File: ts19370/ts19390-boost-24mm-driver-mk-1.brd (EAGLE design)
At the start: 20 x 20 mm, 14 parts, among them U1 TINY85, U2 AMC7135SOT-89, U3 AMC7135SOT-89, U4 AMC7135SOT-89, U5 AMC7135SOT-89

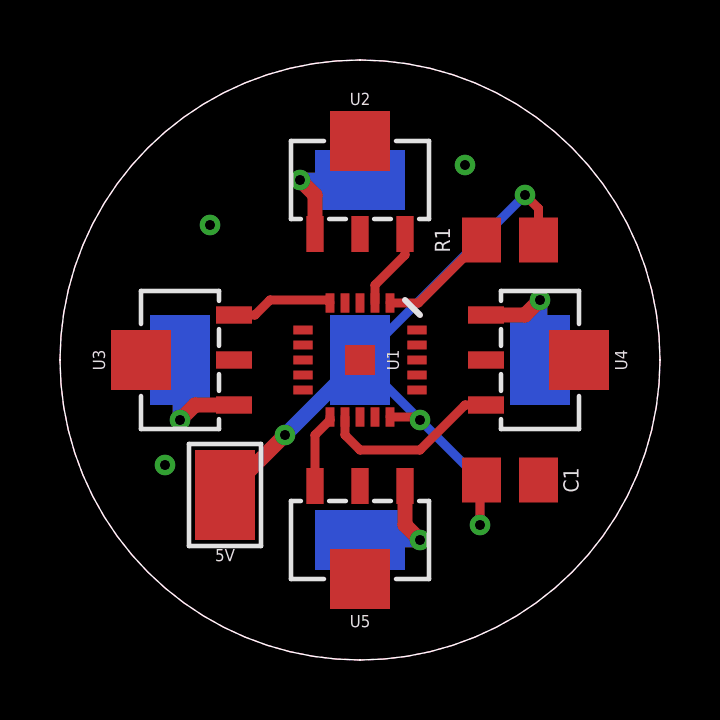
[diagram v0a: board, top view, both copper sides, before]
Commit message: faaaabulous flashlight in progress
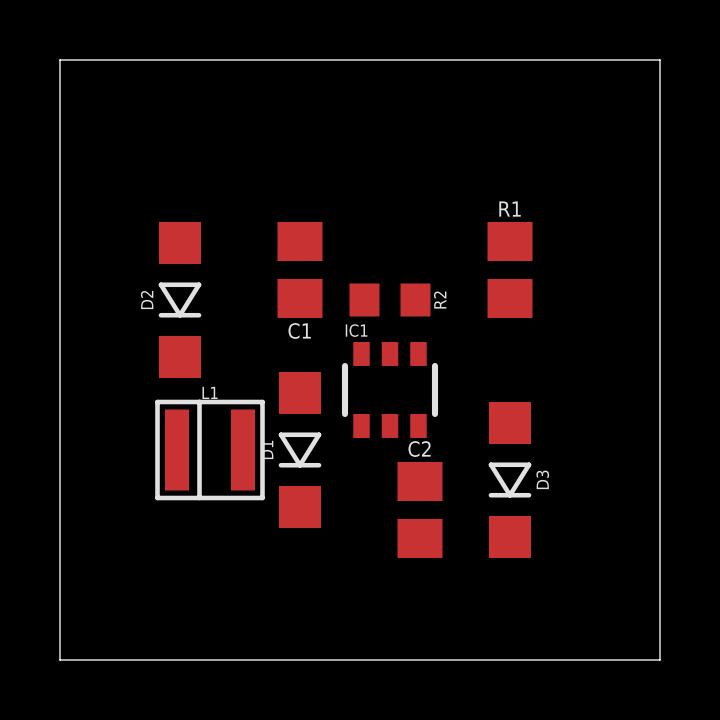
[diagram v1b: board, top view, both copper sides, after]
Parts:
- removed +, 5V, B-, G-, R-, W-: M01SMD_2X3MM, A_butts:1X01_SMD_2X3MM
- removed GND: M01NOT-A-VIA-NOPE, A_butts:1X01_NOSILK_NOSTOP
- removed U1: TINY85, A_butts:QFN20
- removed U2, U3, U4, U5: AMC7135SOT-89, A_butts:SOT89
- added C2: 1uF, A_butts:C0805
- added D1, D2: B340A, A_butts:SOD123
- added D3: 10V, A_butts:SOD123
- added IC1: TS19370, A_butts:SOT26
- added L1: 22uH, A_butts:TAIYO-YUDEN-30XX
- added R2: 10-30k, A_butts:R0603
- C1: value 10uF -> 1uF
- R1: value 100k -> 4.7R
- moved C1 9.90 mm to (8.00, 13.0), turned to 90 degrees
- moved R1 1.00 mm to (15.0, 13.0), turned to 270 degrees
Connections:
- removed net 5V: +.P$1, 5V.P$1, C1.1, R1.1, U1.15
- removed net BLUE-: B-.P$1, U4.1
- removed net BLUEPWM: U1.12, U4.3
- removed net GREEN-: G-.P$1, U3.1
- removed net GREENPWM: U1.5, U3.3
- removed net RED-: R-.P$1, U2.1
- removed net REDPWM: U1.2, U2.3
- removed net WHITE-: U5.1, W-.P$1
- removed net WHITEPWM: U1.11, U5.3
- new net BATT+: D2.A
- new net LED+: C2.1, D1.C, D3.C
- new net LED-: D3.A, IC1.3, R1.2
- new net N$2: IC1.4, R2.1
- new net VCC: C1.1, D2.C, IC1.6, L1.1, R2.2
- net GND: now also C2.2, IC1.2, R1.1; no longer GND.P$1, U1.0, U1.8, U2.2, U2.4, U3.2, U3.4, U4.2, U4.4, U5.2, U5.4
- net N$1: now also D1.A, IC1.1, L1.2; no longer R1.2, U1.1
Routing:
- net 5V: track 25.5 -> 0.00 mm, vias 4 -> 0
- net BLUEPWM: track 6.13 -> 0.00 mm
- net RED-: track 4.01 -> 0.00 mm, vias 1 -> 0
- net BLUE-: track 4.01 -> 0.00 mm, vias 1 -> 0
- net WHITE-: track 4.01 -> 0.00 mm, vias 1 -> 0
- net GREEN-: track 4.01 -> 0.00 mm, vias 1 -> 0
- net N$1: track 3.92 -> 0.00 mm
- net GREENPWM: track 3.45 -> 0.00 mm
- net REDPWM: track 2.71 -> 0.00 mm
- net WHITEPWM: track 2.51 -> 0.00 mm
- removed copper zone on layer 1, net GND
- removed copper zone on layer 16, net GND
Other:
- outline, holes or cut-outs redrawn
